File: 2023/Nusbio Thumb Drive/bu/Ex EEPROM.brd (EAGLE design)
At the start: 68 x 58 mm, 8 parts

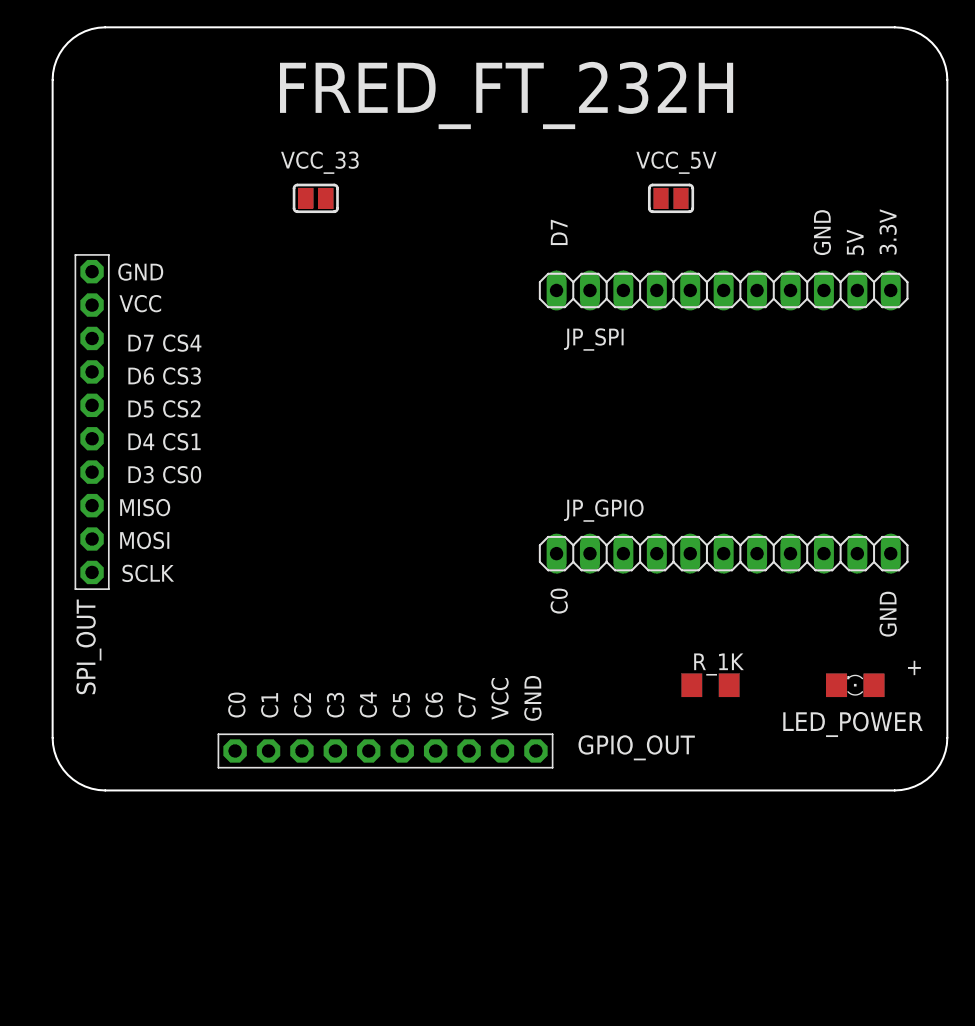
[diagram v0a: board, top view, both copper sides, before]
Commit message: new ft232 board 2023
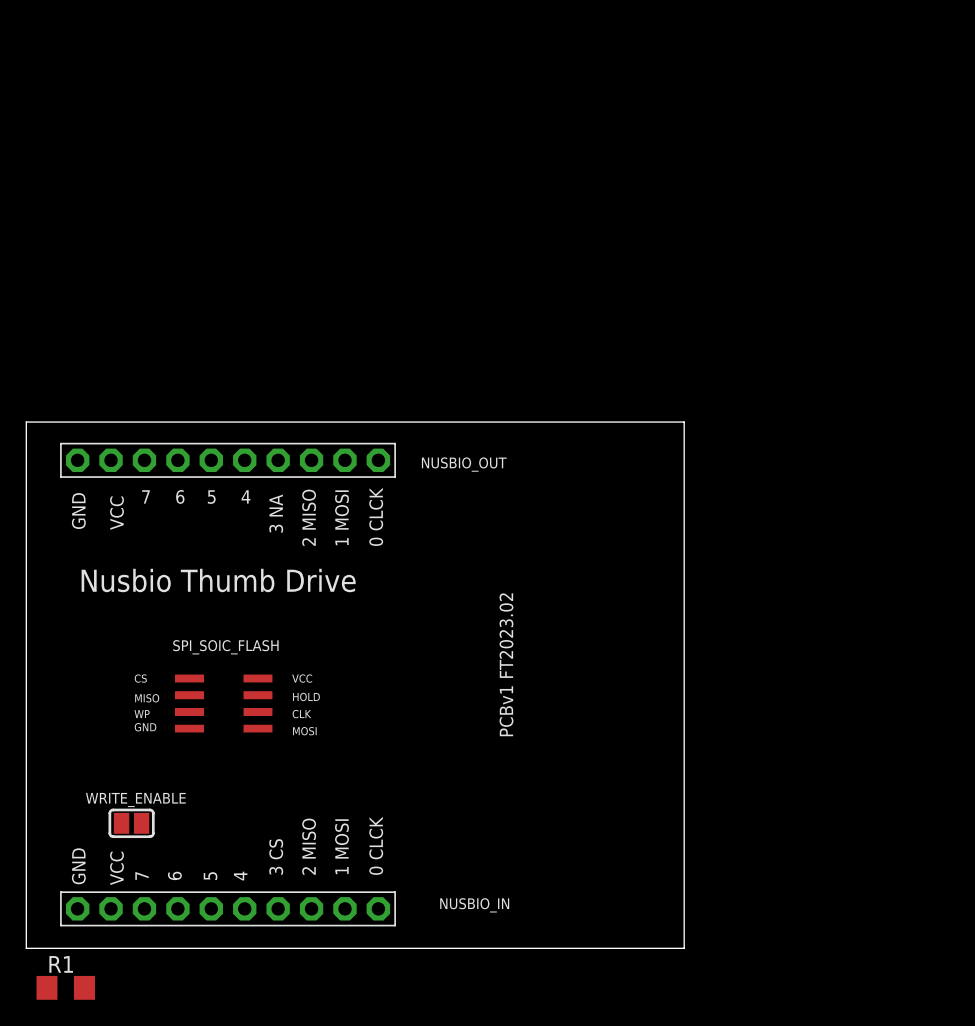
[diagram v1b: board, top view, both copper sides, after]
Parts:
- removed GPIO_OUT, SPI_OUT: PINHD-1X10, adafruit:1X10-BIG
- removed JP_GPIO, JP_SPI: (no value), pinhead:1X11
- removed LED_POWER: (no value), adafruit:1206
- removed R_1K: (no value), adafruit:R1206
- removed VCC_33, VCC_5V: (no value), microbuilder:SOLDERJUMPER_REFLOW
- added NUSBIO_IN, NUSBIO_OUT: PINHD-1X10, adafruit:1X10-BIG
- added R1: (no value), adafruit:R1206
- added SPI_SOIC_FLASH: 25AA080SN, microchip:SO-08
- added WRITE_ENABLE: (no value), microbuilder:SOLDERJUMPER_REFLOW
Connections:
- removed net C0: GPIO_OUT.10, JP_GPIO.1
- removed net C1: GPIO_OUT.9, JP_GPIO.2
- removed net C2: GPIO_OUT.8, JP_GPIO.3
- removed net C3: GPIO_OUT.7, JP_GPIO.4
- removed net C4: GPIO_OUT.6, JP_GPIO.5
- removed net C5: GPIO_OUT.5, JP_GPIO.6
- removed net C6: GPIO_OUT.4, JP_GPIO.7
- removed net C7: GPIO_OUT.3, JP_GPIO.8
- removed net D0_SCLK: JP_SPI.8, SPI_OUT.10
- removed net D1_MOSI: JP_SPI.7, SPI_OUT.9
- removed net D2_MISO: JP_SPI.6, SPI_OUT.8
- removed net D3_CS0: JP_SPI.5, SPI_OUT.7
- removed net D4_CS1: JP_SPI.4, SPI_OUT.6
- removed net D5_CS2: JP_SPI.3, SPI_OUT.5
- removed net D6_CS3: JP_SPI.2, SPI_OUT.4
- removed net D7_CS4: JP_SPI.1, SPI_OUT.3
- removed net VCC_33: JP_SPI.11, VCC_33.2
- removed net VCC_5: JP_SPI.10, LED_POWER.A, VCC_5V.2
- new net CS: NUSBIO_IN.4, NUSBIO_OUT.4, SPI_SOIC_FLASH.1
- new net GPIO5: NUSBIO_IN.5, NUSBIO_OUT.5
- new net GPIO6: NUSBIO_IN.6, NUSBIO_OUT.6
- new net GPIO7: NUSBIO_IN.7, NUSBIO_OUT.7
- new net GPIO8: NUSBIO_IN.8, NUSBIO_OUT.8
- new net MISO: NUSBIO_IN.3, NUSBIO_OUT.3, SPI_SOIC_FLASH.2
- new net MOSI: NUSBIO_IN.2, NUSBIO_OUT.2, SPI_SOIC_FLASH.5
- new net SCK: NUSBIO_IN.1, NUSBIO_OUT.1, SPI_SOIC_FLASH.6
- net GND: now also NUSBIO_IN.10, NUSBIO_OUT.10, SPI_SOIC_FLASH.4; no longer GPIO_OUT.1, JP_GPIO.11, JP_SPI.9, R_1K.1, SPI_OUT.1
- net N$1: now also SPI_SOIC_FLASH.3, WRITE_ENABLE.2; no longer LED_POWER.C, R_1K.2
- net VCC: now also NUSBIO_IN.9, NUSBIO_OUT.9, SPI_SOIC_FLASH.7, SPI_SOIC_FLASH.8, WRITE_ENABLE.1; no longer GPIO_OUT.2, SPI_OUT.2, VCC_33.1, VCC_5V.1
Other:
- board size 68 x 58 mm -> 50 x 40 mm
- board text added: "0 CLCK"
- board text added: "1 MOSI"
- board text added: "2 MISO"
- board text added: "3 CS"
- board text added: "3 NA"
- board text added: "4"
- board text added: "5"
- board text added: "6"
- board text added: "7"
- board text added: "CLK"
- board text added: "CS"
- board text added: "HOLD"
- board text added: "MadeInTheUSB.net"
- board text added: "Nusbio Thumb Drive"
- board text added: "PCBv1 FT2023.02"
- board text added: "WP"
- board text removed: "+"
- board text removed: "3.3V"
- board text removed: "5V"
- board text removed: "C0"
- board text removed: "C1"
- board text removed: "C2"
- board text removed: "C3"
- board text removed: "C4"
- board text removed: "C5"
- board text removed: "C6"
- board text removed: "C7"
- board text removed: "D3 CS0"
- board text removed: "D4 CS1"
- board text removed: "D5 CS2"
- board text removed: "D6 CS3"
- board text removed: "D7"
- board text removed: "D7 CS4"
- board text removed: "FRED_FT_232H"
- board text removed: "PCBv1 - 2023.02"
- board text removed: "SCLK"
- board text removed: "www.FredericTorres.com"
